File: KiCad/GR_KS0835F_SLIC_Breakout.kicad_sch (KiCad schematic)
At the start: 25 parts, among them J1 USB_B_Micro, J2 Conn_01x03, J3 Conn_01x07, J4 Conn_01x07, U1 ATtiny x04/x14, U2 CH340G, Y1 12MHz

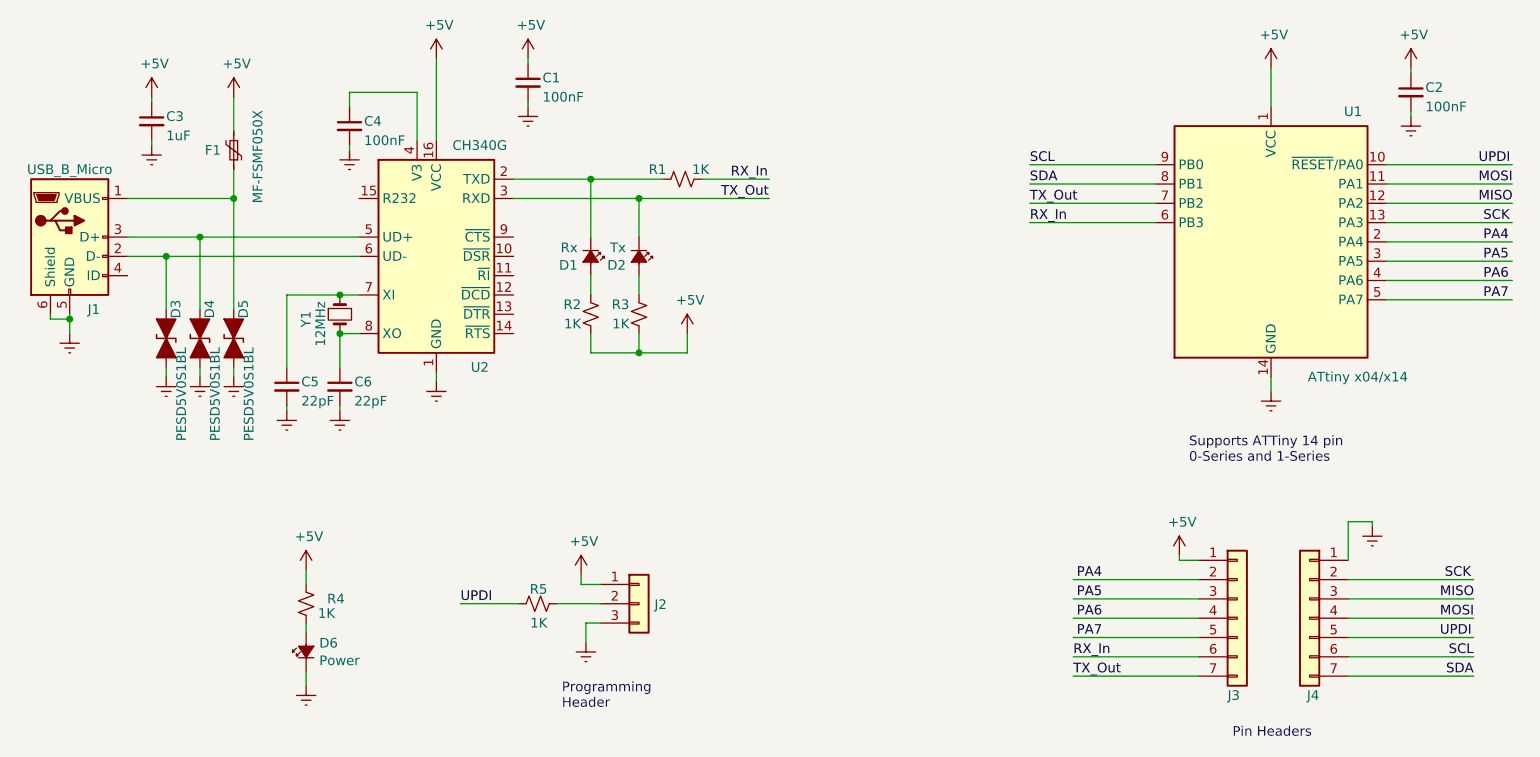
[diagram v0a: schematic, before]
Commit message: Add files via upload
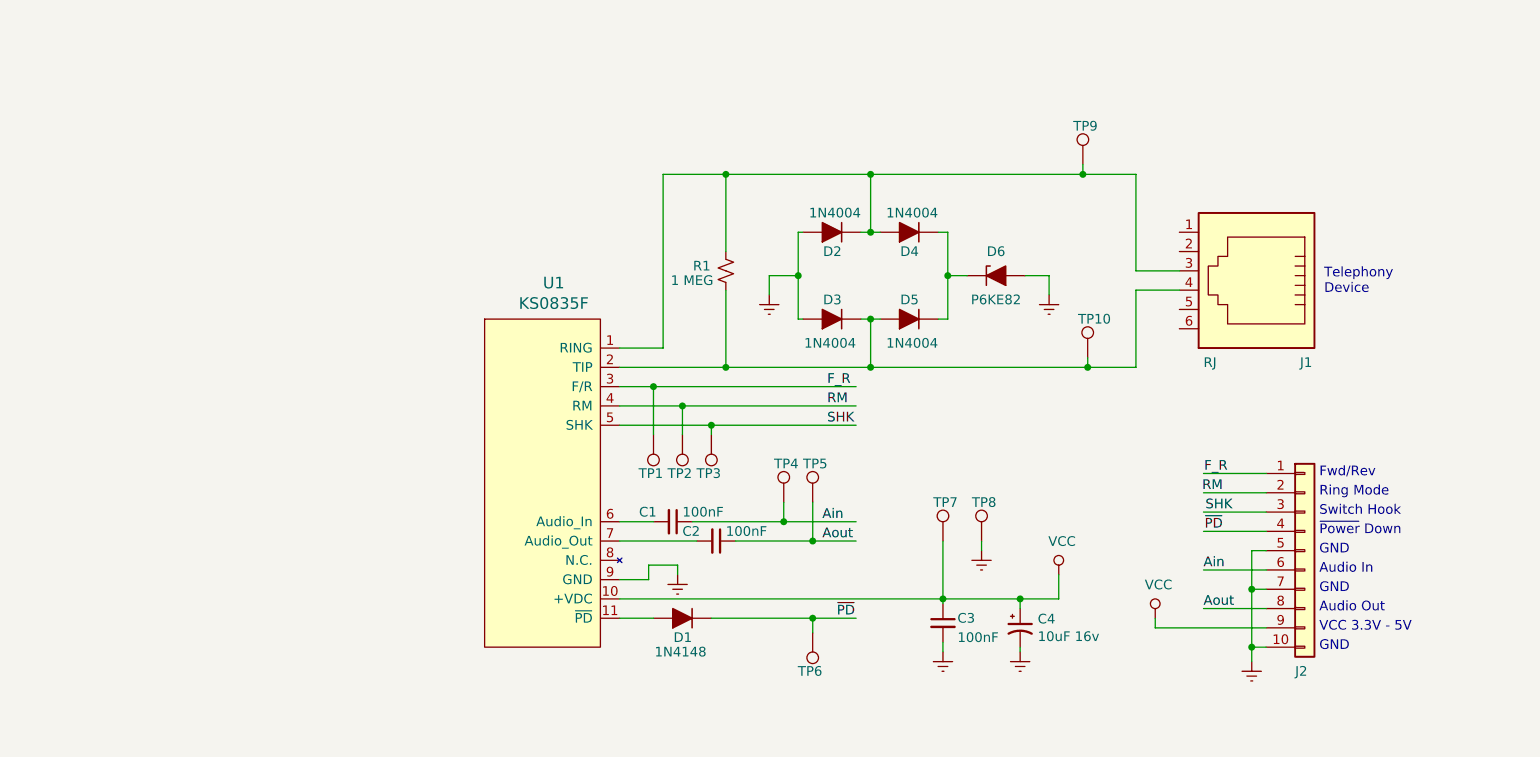
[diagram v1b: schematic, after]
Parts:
- removed C1, C2, C4: 100nF, Capacitor_SMD:C_0805_2012Metric_Pad1.15x1.40mm_HandSolder, symbol GR_ATTiny_xx4_USB-rescue:C_Small-Device
- removed C3: 1uF, Capacitor_SMD:C_0805_2012Metric_Pad1.15x1.40mm_HandSolder, symbol GR_ATTiny_xx4_USB-rescue:C_Small-Device
- removed C5, C6: 22pF, Capacitor_SMD:C_0805_2012Metric_Pad1.15x1.40mm_HandSolder, symbol GR_ATTiny_xx4_USB-rescue:C_Small-Device
- removed D1: Rx, LED_SMD:LED_0805_2012Metric_Pad1.15x1.40mm_HandSolder, symbol GR_ATTiny_xx4_USB-rescue:LED_Small_ALT-Device
- removed D2: Tx, LED_SMD:LED_0805_2012Metric_Pad1.15x1.40mm_HandSolder, symbol GR_ATTiny_xx4_USB-rescue:LED_Small_ALT-Device
- removed D3, D4, D5: PESD5V0S1BL, _Custom_Footprints:SOD-882, symbol GR_ATTiny_xx4_USB-rescue:D_TVS_ALT-Device
- removed D6: Power, LED_SMD:LED_0805_2012Metric_Pad1.15x1.40mm_HandSolder, symbol GR_ATTiny_xx4_USB-rescue:LED_Small_ALT-Device
- removed F1: MF-FSMF050X, Resistor_SMD:R_0603_1608Metric_Pad1.05x0.95mm_HandSolder, symbol GR_ATTiny_xx4_USB-rescue:Polyfuse_Small-Device
- removed J1: USB_B_Micro, Connector_USB:USB_Micro-B_Amphenol_10103594-0001LF_Horizontal, symbol GR_ATTiny_xx4_USB-rescue:USB_B_Micro-Connector
- removed J2: Conn_01x03, Connector_PinHeader_2.54mm:PinHeader_1x03_P2.54mm_Vertical, symbol GR_ATTiny_xx4_USB-rescue:Conn_01x03-Connector_Generic
- removed J3, J4: Conn_01x07, Connector_PinHeader_2.54mm:PinHeader_1x07_P2.54mm_Vertical, symbol GR_ATTiny_xx4_USB-rescue:Conn_01x07-Connector_Generic
- removed R1, R2, R3, R4, R5: 1K, Resistor_SMD:R_0805_2012Metric_Pad1.15x1.40mm_HandSolder, symbol GR_ATTiny_xx4_USB-rescue:R_Small_US-Device
- removed U1: ATtiny x04/x14, Package_SO:SOIC-14_3.9x8.7mm_P1.27mm, symbol GR_ATTiny_xx4_USB-rescue:ATtiny804-SS-MCU_Microchip_ATtiny
- removed U2: CH340G, Package_SO:SOIC-16_3.9x9.9mm_P1.27mm, symbol GR_ATTiny_xx4_USB-rescue:CH340G-Interface_USB
- removed Y1: 12MHz, Crystal:Crystal_SMD_HC49-SD_HandSoldering, symbol GR_ATTiny_xx4_USB-rescue:Crystal_Small-Device
- added C1, C2, C3: 100nF, Capacitor_THT:C_Disc_D4.3mm_W1.9mm_P5.00mm, symbol Device:C_Small
- added C4: 10uF 16v, Capacitor_THT:CP_Radial_D8.0mm_P5.00mm, symbol GR_KS0835F_SLIC_Breakout-rescue:CP1_Small-Device
- added D1: 1N4148, Diode_THT:D_DO-35_SOD27_P7.62mm_Horizontal, symbol GR_KS0835F_SLIC_Breakout-rescue:D_ALT-Device
- added D2, D3, D4, D5: 1N4004, Diode_THT:D_DO-41_SOD81_P10.16mm_Horizontal, symbol GR_KS0835F_SLIC_Breakout-rescue:D_ALT-Device
- added D6: P6KE82, Diode_THT:D_DO-15_P12.70mm_Horizontal, symbol GR_KS0835F_SLIC_Breakout-rescue:D_Zener_ALT-Device
- added J1: RJ, footprints:RJ_6p6c, symbol Connector:RJ12
- added J2: Conn_01x10, Connector_PinHeader_2.54mm:PinHeader_1x10_P2.54mm_Vertical, symbol Connector_Generic:Conn_01x10
- added R1: 1 MEG, Resistor_THT:R_Axial_DIN0309_L9.0mm_D3.2mm_P12.70mm_Horizontal, symbol Device:R_Small_US
- added TP1, TP10, TP2, TP3, TP4, TP5, TP6, TP7, TP8, TP9: TestPoint, TestPoint:TestPoint_Pad_D1.0mm, symbol Connector:TestPoint
- added U1: KS0835F, footprints:KS0835F, symbol KS0835F:KS0835F
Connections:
- net GNDREF: now also C3.2, C4.2, D2.2 (A), D3.2 (A), D6.2 (A), J2.10 (Pin_10), J2.5 (Pin_5), J2.7 (Pin_7), TP8.1, U1.9 (GND)
- new net: D2.1 (K), D4.2 (A), J1.3, R1.2, TP9.1, U1.1 (RING)
- new net: D3.1 (K), D5.2 (A), J1.4, R1.1, TP10.1, U1.2 (TIP)
- new net: D1.2 (A), U1.11 (~{PD})
- new net: C1.2, U1.6 (Audio_In)
- new net: C2.2, U1.7 (Audio_Out)
- new net: D4.1 (K), D5.1 (K), D6.1 (K)
- new net Ain: C1.1, J2.6 (Pin_6), TP4.1
- new net Aout: C2.1, J2.8 (Pin_8), TP5.1
- new net F_R: J2.1 (Pin_1), TP1.1, U1.3 (F/R)
- new net RM: J2.2 (Pin_2), TP2.1, U1.4 (RM)
- new net SHK: J2.3 (Pin_3), TP3.1, U1.5 (SHK)
- new net VCC: C3.1, C4.1, J2.9 (Pin_9), TP7.1, U1.10 (+VDC)
- new net ~{PD}: D1.1 (K), J2.4 (Pin_4), TP6.1
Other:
- note added: "Audio In"
- note added: "Audio Out"
- note added: "Fwd/Rev"
- note added: "GND"
- note added: "Ring Mode"
- note added: "Switch Hook"
- note added: "Telephony Device"
- note added: "VCC 3.3V - 5V"
- note added: "~{Power} Down"
- note removed: "Pin Headers"
- note removed: "Programming Header"
- note removed: "Supports ATTiny 14 pin 0-Series and 1-Series"
- title: ATTiny 14 pin 0-Series and 1-Series USB Breakout -> KS0835F SLIC Breakout
